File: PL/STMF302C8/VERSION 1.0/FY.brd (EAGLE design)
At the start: 70 x 69 mm, 55 parts, among them J1 CON-SD-CARD_MICROSD-2908-05, J2 Flash Programming, U1 AS72652-BLGT, U2 AS72653-BLGT, U3 STM32F302C8T6, U4 AS72651-BLGT, U5 AMS1117-3.3, U6 4MB Flash, X1 JST-XH-04-PIN-LONG-PAD, Y2 ABM2B-8.000MHZ-10-1-U-T

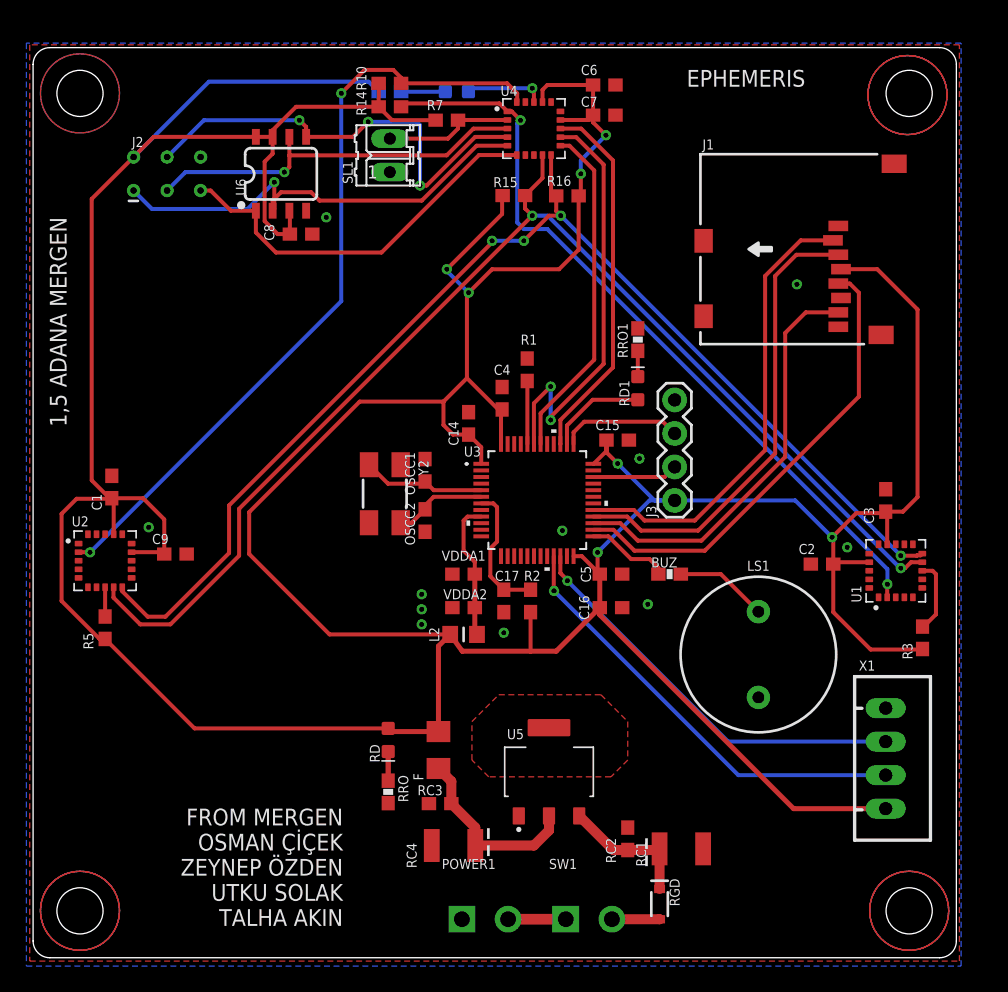
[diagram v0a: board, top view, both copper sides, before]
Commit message: Version 2.0 was relased by brain.dll
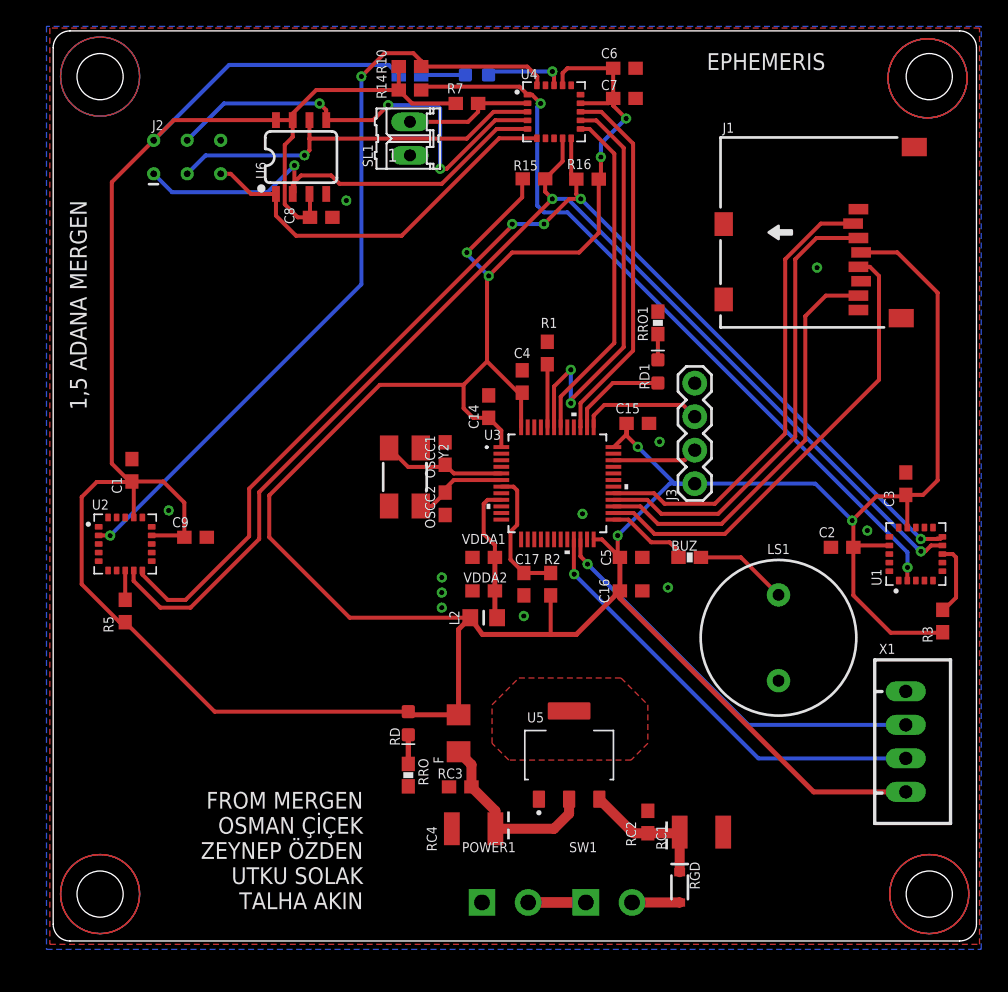
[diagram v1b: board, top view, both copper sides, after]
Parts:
- moved RC4 1.98 mm to (33.4, 9.78)
- moved BUZ 1.98 mm to (49.8, 30.4)
- moved C17 1.98 mm to (37.2, 28.3)
- moved C3 1.98 mm to (66.2, 35.9)
- moved C4 1.98 mm to (37.1, 43.7)
- moved C5 1.98 mm to (45.3, 30.4)
- moved C8 1.98 mm to (21.8, 56.1)
- moved J1 1.98 mm to (66.4, 55.0)
- moved J3 1.98 mm to (50.2, 35.9)
- moved LS1 1.98 mm to (56.5, 24.3)
- moved OSCC2 1.98 mm to (31.2, 34.4)
- moved R15 1.98 mm to (38.0, 59.1)
- moved R16 1.98 mm to (42.0, 59.0)
- moved R2 1.98 mm to (39.2, 28.3)
- moved RD1 1.98 mm to (47.4, 44.5)
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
